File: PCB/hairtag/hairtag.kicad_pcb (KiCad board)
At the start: 2 copper layers, 23 x 23 mm, 17 parts, among them U1 ESP32-C3FH4, X1 XL2EL89CPI-111YLC-40M

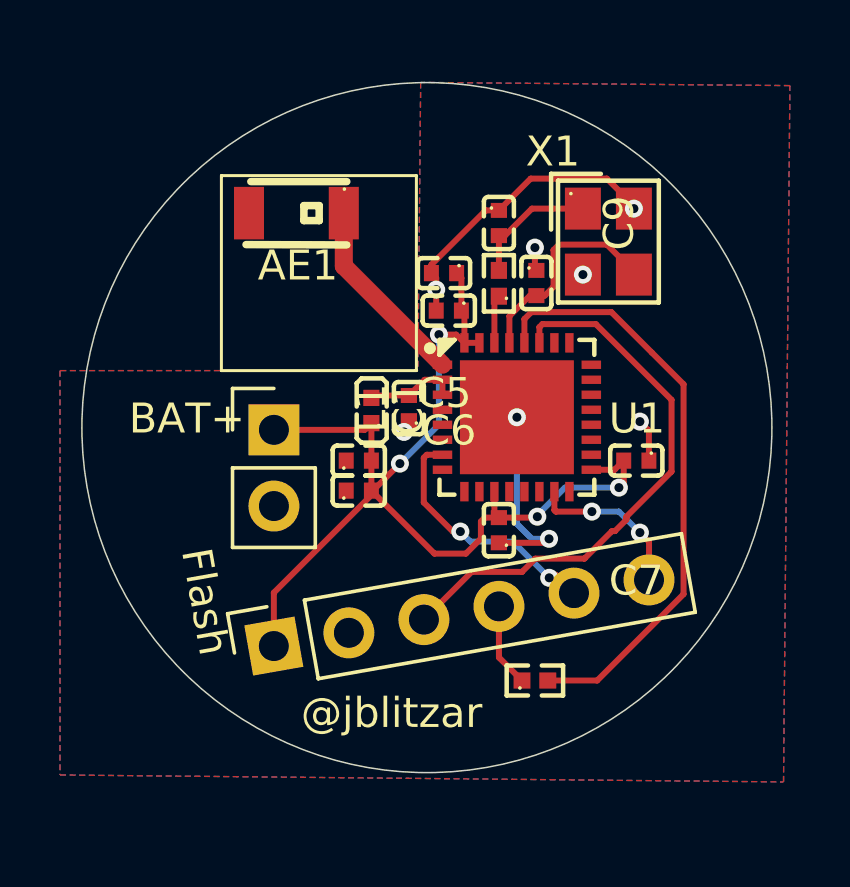
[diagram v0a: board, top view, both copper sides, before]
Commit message: misc stuff
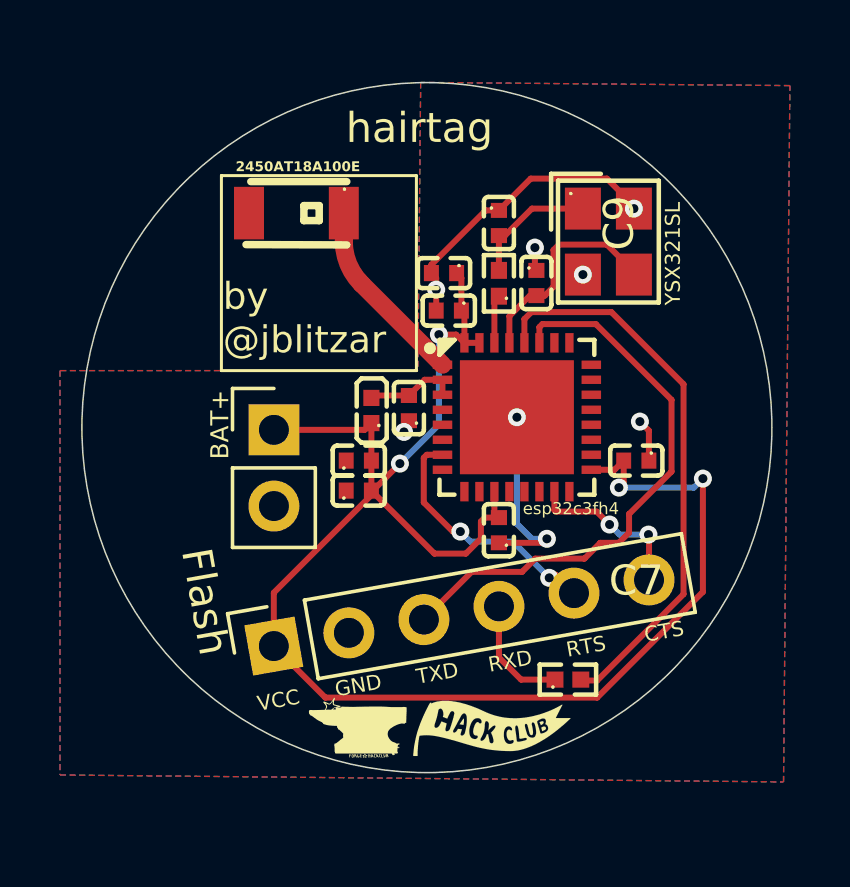
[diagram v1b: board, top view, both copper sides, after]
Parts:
- moved R1 1.10 mm to (59.8, 63.8)
- renumbered AE1 to 2450AT18A100E, X1 to YSX321SL, U1 to esp32c3fh4
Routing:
- net /VCC: track 35.7 -> 54.3 mm
- net Net-(U1-U0TXD): track 19.9 -> 18.8 mm
- net /RXD: track 2.79 -> 3.88 mm
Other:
- board text added: "CTS"
- board text added: "GND"
- board text added: "RTS"
- board text added: "RXD"
- board text added: "TXD"
- board text added: "VCC"
- board text added: "by @jblitzar"
- board text added: "hairtag"
- board text removed: "@jblitzar"

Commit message: readme stuff
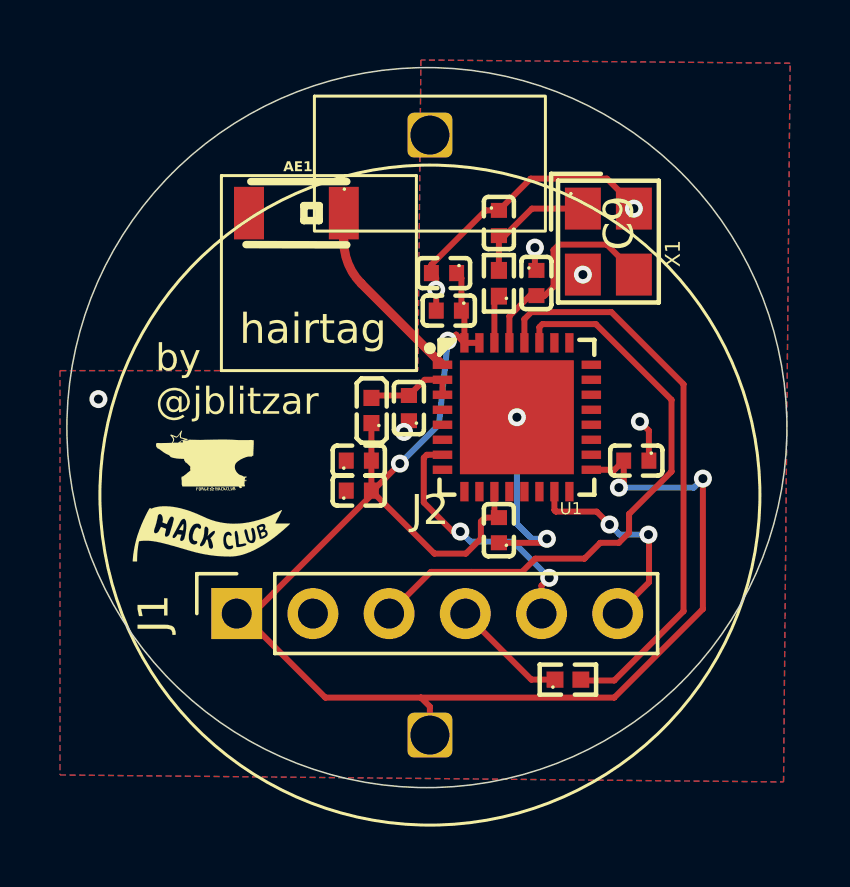
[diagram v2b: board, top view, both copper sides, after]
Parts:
- removed BAT+: BAT, Connector_PinHeader_2.54mm:PinHeader_1x02_P2.54mm_Vertical
- removed Flash: Flash, Connector_PinSocket_2.54mm:PinSocket_1x06_P2.54mm_Vertical
- added J1: Flash, Connector_PinSocket_2.54mm:PinSocket_1x06_P2.54mm_Vertical, F.Cu at (48.8, 61.6)
- added J2: BAT, cr2032_holder:Untitled, F.Cu at (55.2, 58.6)
- renumbered 2450AT18A100E to AE1, esp32c3fh4 to U1, YSX321SL to X1
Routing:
- net /CTS: track 5.61 -> 7.16 mm
- net /TXD: track 19.1 -> 20.1 mm
- net /VCC: track 54.3 -> 53.6 mm
- net GND: vias 8 -> 9
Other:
- board size 23 x 23 mm -> 24 x 24 mm
- board text removed: "CTS"
- board text removed: "GND"
- board text removed: "RTS"
- board text removed: "RXD"
- board text removed: "TXD"
- board text removed: "VCC"
